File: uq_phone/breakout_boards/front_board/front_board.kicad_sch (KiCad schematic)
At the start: 61 parts, among them J5 FI-RE51S-HF-R1500, J9 541324562, SW1 SKTAAAE010, SW10 SKTAAAE010, SW11 SKTAAAE010, SW12 SKTAAAE010, SW13 SKTAAAE010, SW14 SKTAAAE010, SW15 SKTAAAE010, SW16 SKTAAAE010, SW17 SKTAAAE010, SW18 SKTAAAE010, SW19 SKTAAAE010, SW2 SKTAAAE010, SW20 SKTAAAE010, SW21 SKTAAAE010, SW22 SKTAAAE010, SW23 SKTAAAE010, SW24 SKTAAAE010, SW25 SKTAAAE010, SW27 SKTAAAE010, SW29 SKTAAAE010, SW3 SKTAAAE010, SW31 SKTAAAE010, SW33 SKTAAAE010, SW34 SKTAAAE010, SW35 SKTAAAE010, SW36 SKTAAAE010, SW37 SKTAAAE010, SW38 SKTAAAE010, SW39 SKTAAAE010, SW4 SKTAAAE010, SW40 SKTAAAE010, SW41 SKTAAAE010, SW42 SKTAAAE010, SW43 SKSCLCE010, SW44 SKSCLCE010, SW45 SKSCLCE010, SW5 SKTAAAE010, SW6 SKTAAAE010, SW7 SKTAAAE010, SW8 SKTAAAE010, SW9 SKTAAAE010

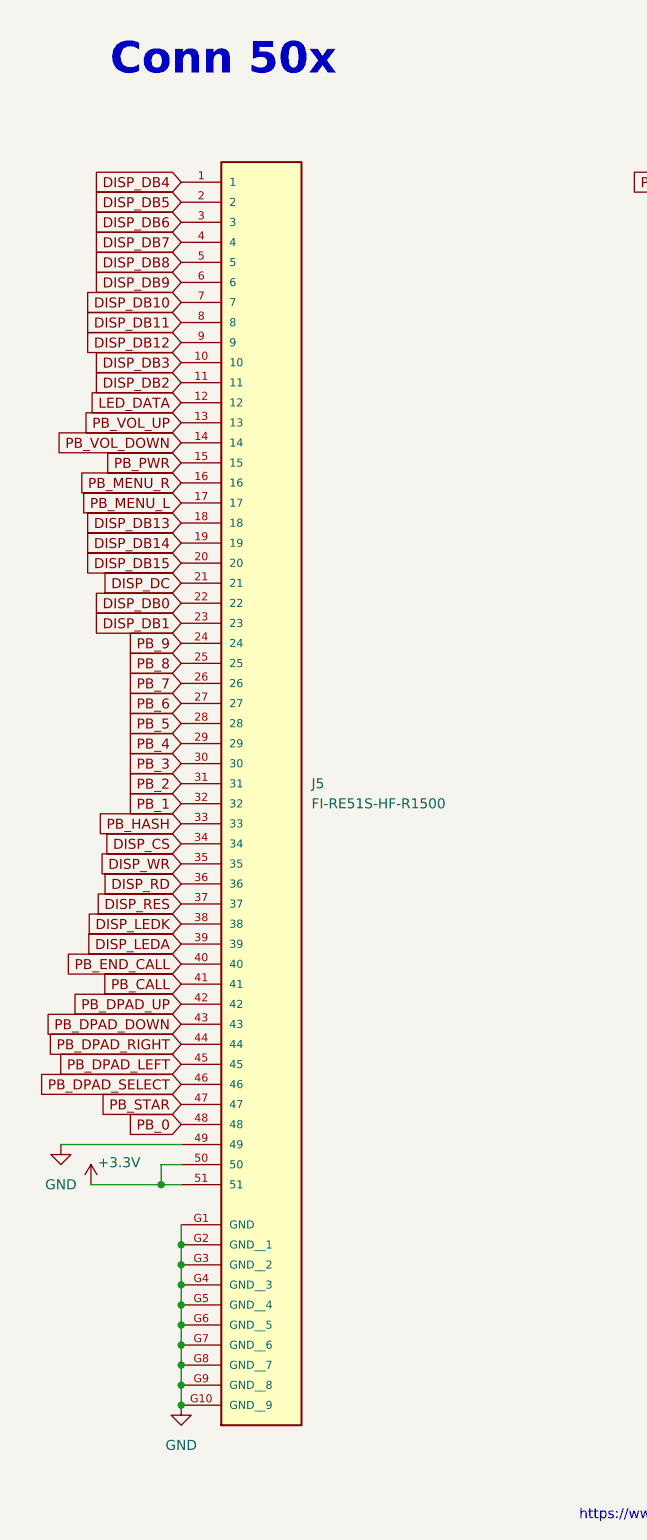
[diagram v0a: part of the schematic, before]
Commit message: Update Various Connectors
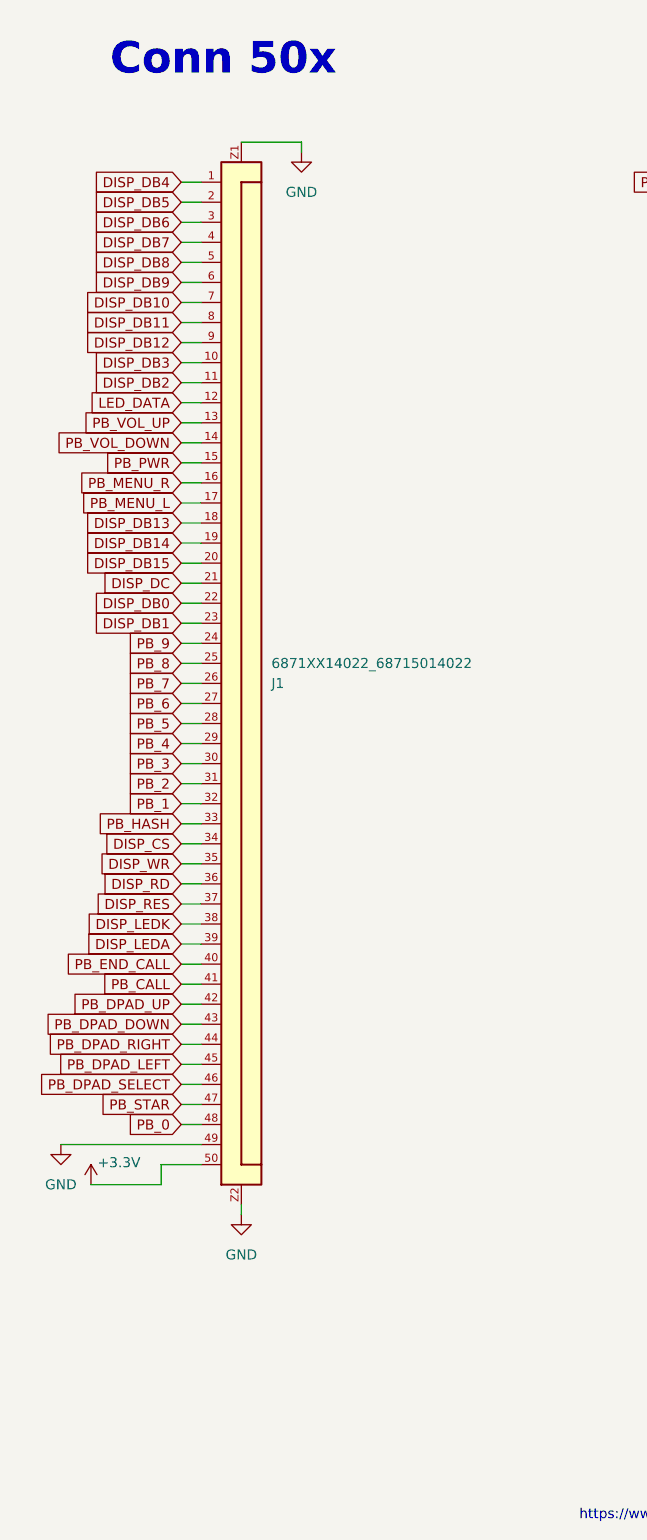
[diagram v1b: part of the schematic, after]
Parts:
- removed J5: FI-RE51S-HF-R1500, FI-RE51S-HF-R1500:JAE_FI-RE51S-HF-R1500, symbol FI-RE51S-HF-R1500:FI-RE51S-HF-R1500
- added J1: 6871XX14022_68715014022, 6871XX14022_68715014022:68715014022, symbol 6871XX14022_68715014022:6871XX14022_68715014022
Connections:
- net +3.3V: now also J1.50
- net DISP_CS: now also J1.34
- net DISP_DB0: now also J1.22
- net DISP_DB1: now also J1.23
- net DISP_DB10: now also J1.7
- net DISP_DB11: now also J1.8
- net DISP_DB12: now also J1.9
- net DISP_DB13: now also J1.18
- net DISP_DB14: now also J1.19
- net DISP_DB15: now also J1.20
- net DISP_DB2: now also J1.11
- net DISP_DB3: now also J1.10
- net DISP_DB4: now also J1.1
- net DISP_DB5: now also J1.2
- net DISP_DB6: now also J1.3
- net DISP_DB7: now also J1.4
- net DISP_DB8: now also J1.5
- net DISP_DB9: now also J1.6
- net DISP_DC: now also J1.21
- net DISP_LEDA: now also J1.39
- net DISP_LEDK: now also J1.38
- net DISP_RD: now also J1.36
- net DISP_RES: now also J1.37
- net DISP_WR: now also J1.35
- net GND: now also J1.49, J1.Z1, J1.Z2
- net LED_DATA: now also J1.12
- net PB_0: now also J1.48
- net PB_1: now also J1.32
- net PB_2: now also J1.31
- net PB_3: now also J1.30
- net PB_4: now also J1.29
- net PB_5: now also J1.28
- net PB_6: now also J1.27
- net PB_7: now also J1.26
- net PB_8: now also J1.25
- net PB_9: now also J1.24
- net PB_CALL: now also J1.41
- net PB_DPAD_DOWN: now also J1.43
- net PB_DPAD_LEFT: now also J1.45
- net PB_DPAD_RIGHT: now also J1.44
- net PB_DPAD_SELECT: now also J1.46
- net PB_DPAD_UP: now also J1.42
- net PB_END_CALL: now also J1.40
- net PB_HASH: now also J1.33
- net PB_MENU_L: now also J1.17
- net PB_MENU_R: now also J1.16
- net PB_PWR: now also J1.15
- net PB_STAR: now also J1.47
- net PB_VOL_DOWN: now also J1.14
- net PB_VOL_UP: now also J1.13
